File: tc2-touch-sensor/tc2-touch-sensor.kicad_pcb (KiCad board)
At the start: 2 copper layers, 50.6 x 17.3 mm, 24 parts, among them J301 Screw_Terminal_01x01, J302 Conn_02x03_Odd_Even, J303 Screw_Terminal_01x01, Q301 AO3400A, U301 ME6216A28XG, U302 AT42QT1010-TSHR

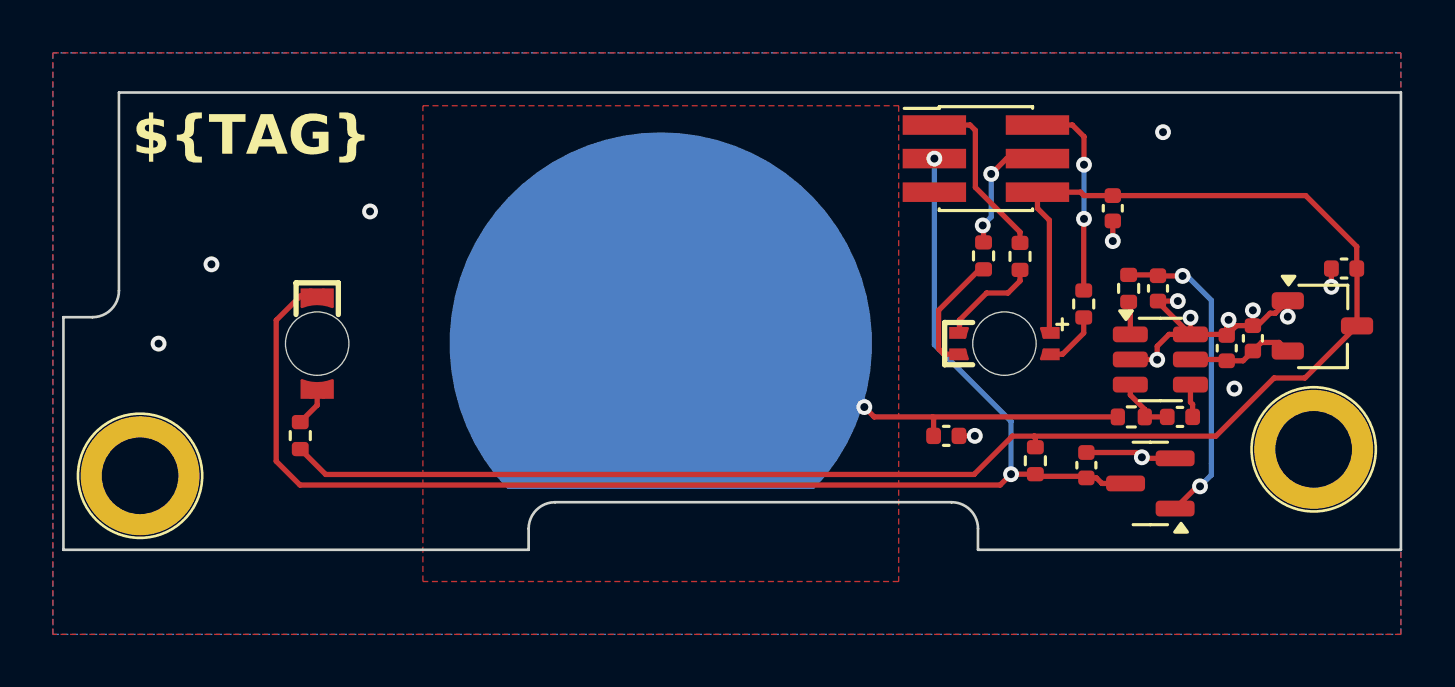
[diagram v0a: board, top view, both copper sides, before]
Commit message: v0.7.3
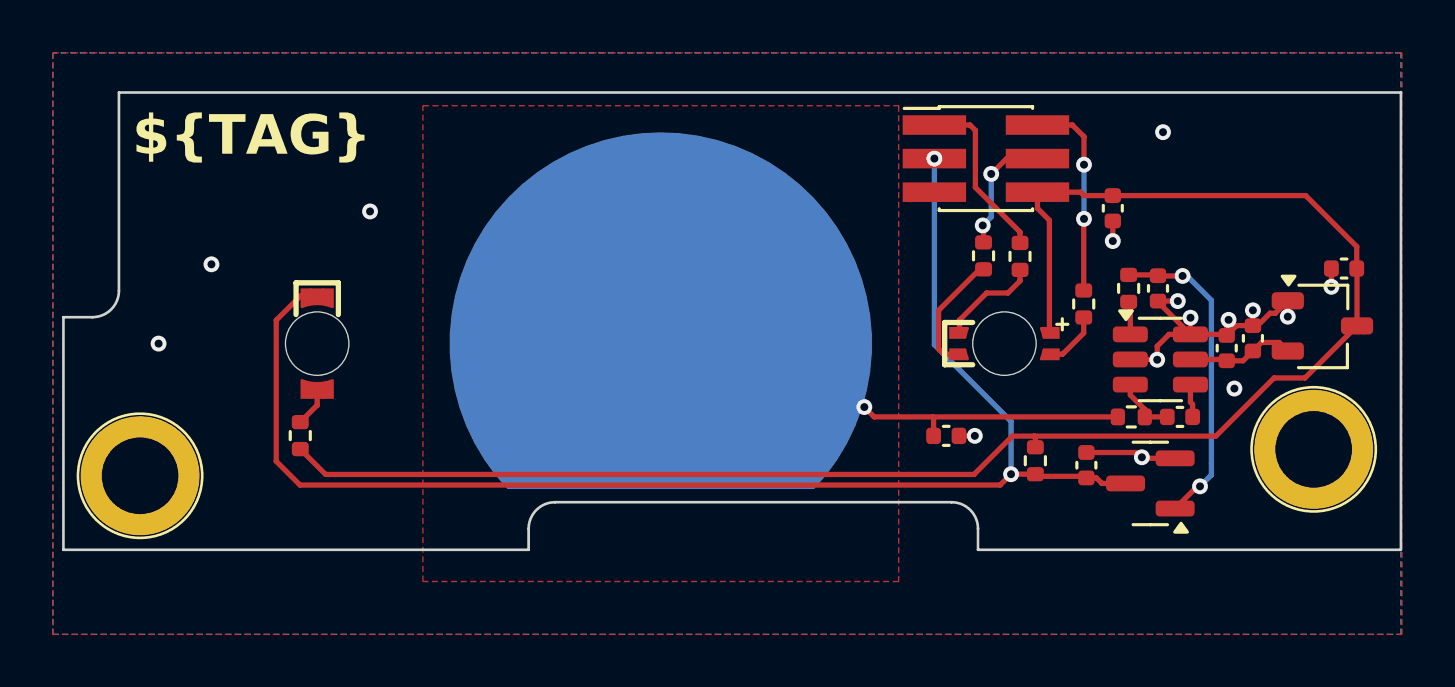
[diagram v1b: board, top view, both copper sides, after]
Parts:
- added REF**: Tab, PCM_kikit:Tab, F.Cu at (17.6, 8.69)
- added REF**: Tab, PCM_kikit:Tab, F.Cu at (19.7, -9.53)
- added REF**: Tab, PCM_kikit:Tab, F.Cu at (28.0, -0.90)
- added REF**: Tab, PCM_kikit:Tab, F.Cu at (-12.1, -9.52)
- added REF**: Tab, PCM_kikit:Tab, F.Cu at (-15.2, 8.73)
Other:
- copper layers 2 -> 6

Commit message: 0.8.0 WIP
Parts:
- R301, R304, R305, R306: value 180R -> 180Ω
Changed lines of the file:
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@@
 			)
 		)
-		(property "Value" "180R"
+		(property "Value" "180Ω"
 			(at 0 1.17 90)
 			(layer "F.Fab")
@@
 			)
 		)
-		(property "Value" "180R"
+		(property "Value" "180Ω"
 			(at 0 1.17 90)
 			(layer "F.Fab")
@@
 			)
 		)
-		(property "Value" "180R"
+		(property "Value" "180Ω"
 			(at 0 1.17 90)
 			(layer "F.Fab")
@@
 			)
 		)
-		(property "Value" "180R"
+		(property "Value" "180Ω"
 			(at 0 1.17 90)
 			(layer "F.Fab")
